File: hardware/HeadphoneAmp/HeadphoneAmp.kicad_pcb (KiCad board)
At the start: 4 copper layers, 100 x 80 mm, 134 parts, among them J1 Preamp Input, J10 Barrel_Jack_Switch, J11 Router Power, J2 Source, J3 1503_02, J4 1503_02, J5 In R, J6 In L, J7 I2S + SPI, J8 Out R, J9 Out L, SW1 SW_SPDT, SW2 Gain Select, U1 NJM2068M, U10 MIC5317, U11 PCM1796DB, U12 ACPL-064L, U13 ACPL-064L, U14 APS1551SZ, U15 ACPL-064L, U16 ACPL-M61L, U2 NJM4556AM, U3 NJM4556AM, U4 NJM5532M, U5 NJM5532M, U6 NJM5532M, U7 L7812ACV, U8 L7912ACV, U9 MCP1755ST-5002xDB

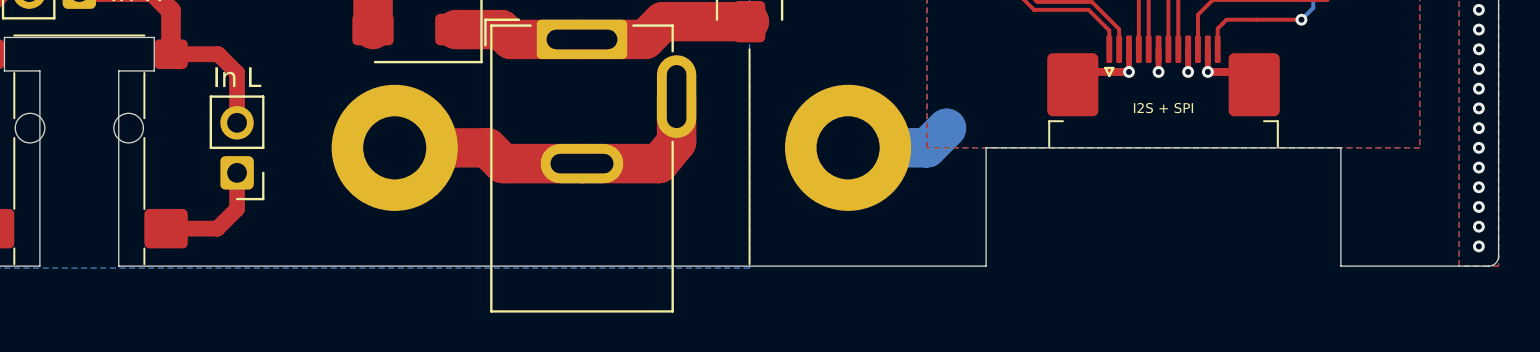
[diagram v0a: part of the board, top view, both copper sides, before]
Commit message: Cleanup in the base board
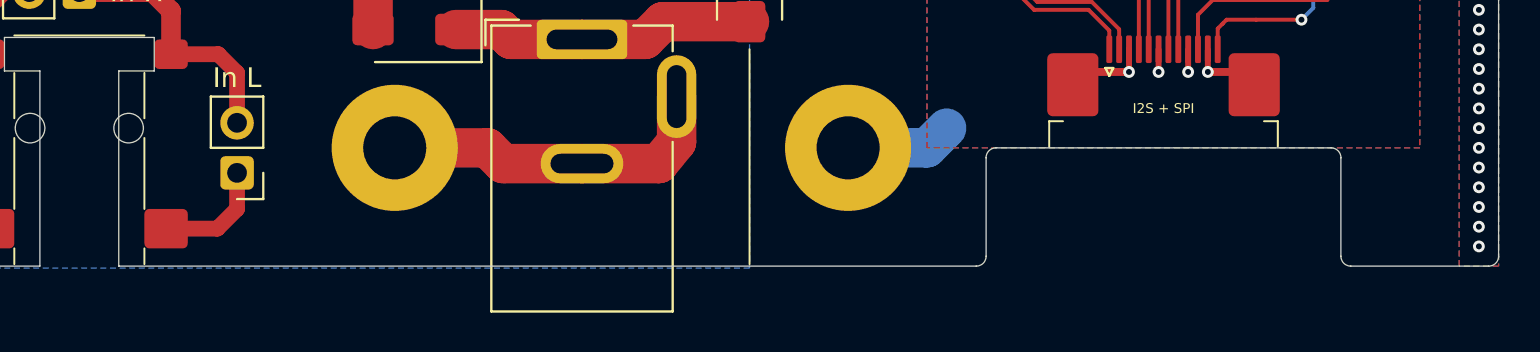
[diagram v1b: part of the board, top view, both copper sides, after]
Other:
- outline, holes or cut-outs redrawn
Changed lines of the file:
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@@
   (gr_arc (start 186 100.5) (mid 186.8 101.3) (end 186 102.1) (layer "Edge.Cuts") (width 0.05))
   (gr_arc locked (start 100.5 140) (mid 100.146447 139.853553) (end 100 139.5) (layer "Edge.Cuts") (width 0.05))
-  (gr_line locked (start 130 140) (end 174 140) (layer "Edge.Cuts") (width 0.05))
+  (gr_line locked (start 130 140) (end 173.5 140) (layer "Edge.Cuts") (width 0.05))
   (gr_arc locked (start 200 139.5) (mid 199.853553 139.853553) (end 199.5 140) (layer "Edge.Cuts") (width 0.05))
   (gr_line locked (start 100.5 60) (end 126 60) (layer "Edge.Cuts") (width 0.05))
-  (gr_line locked (start 192 140) (end 192 134) (layer "Edge.Cuts") (width 0.05))
-  (gr_line locked (start 199.5 140) (end 192 140) (layer "Edge.Cuts") (width 0.05))
+  (gr_arc locked (start 192.5 140) (mid 192.146447 139.853553) (end 192 139.5) (layer "Edge.Cuts") (width 0.05))
+  (gr_line locked (start 192 139.5) (end 192 134.5) (layer "Edge.Cuts") (width 0.05))
+  (gr_line locked (start 199.5 140) (end 192.5 140) (layer "Edge.Cuts") (width 0.05))
   (gr_line (start 172 100.5) (end 186 100.5) (layer "Edge.Cuts") (width 0.05))
+  (gr_arc locked (start 191.5 134) (mid 191.853553 134.146447) (end 192 134.5) (layer "Edge.Cuts") (width 0.05))
+  (gr_arc locked (start 174 134.5) (mid 174.146447 134.146447) (end 174.5 134) (layer "Edge.Cuts") (width 0.05))
   (gr_arc locked (start 100 60.5) (mid 100.146447 60.146447) (end 100.5 60) (layer "Edge.Cuts") (width 0.05))
   (gr_arc (start 172 102.1) (mid 171.2 101.3) (end 172 100.5) (layer "Edge.Cuts") (width 0.05))
   (gr_line locked (start 100 139.5) (end 100 60.5) (layer "Edge.Cuts") (width 0.05))
   (gr_line locked (start 200 139.5) (end 200 60.5) (layer "Edge.Cuts") (width 0.05))
-  (gr_line locked (start 174 134) (end 174 140) (layer "Edge.Cuts") (width 0.05))
+  (gr_line locked (start 174 134.5) (end 174 139.5) (layer "Edge.Cuts") (width 0.05))
   (gr_arc locked (start 199.5 60) (mid 199.853553 60.146447) (end 200 60.5) (layer "Edge.Cuts") (width 0.05))
+  (gr_arc locked (start 174 139.5) (mid 173.853553 139.853553) (end 173.5 140) (layer "Edge.Cuts") (width 0.05))
   (gr_line locked (start 100.5 140) (end 126 140) (layer "Edge.Cuts") (width 0.05))
   (gr_line (start 186 102.1) (end 172 102.1) (layer "Edge.Cuts") (width 0.05))
-  (gr_line locked (start 174 134) (end 192 134) (layer "Edge.Cuts") (width 0.05))
+  (gr_line locked (start 174.5 134) (end 191.5 134) (layer "Edge.Cuts") (width 0.05))
   (gr_line locked (start 130 60) (end 199.5 60) (layer "Edge.Cuts") (width 0.05))
   (gr_text "v2 Strict" (at 113.9 115.8) (layer "F.SilkS")
